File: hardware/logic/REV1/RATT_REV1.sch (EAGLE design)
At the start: 141 parts, among them IC1 MCP73832, IC10 CPC1002N, IC2 TPS2115AIPWRQ1, IC3 MAX98357, IC4 AP2112K-3.3V, IC5 PCA9539PW, IC6 TLP292-4, IC7 CPC1002N, IC8 CPC1002N, IC9 CPC1002N, J10 PHOENIX1803484, J100 RPI-ZERO, J11 PHOENIX1803484, J2 PHOENIX1803426, J3 LiPo, J4 F-1X04-SIP-100-40, J5 4P-2.0, J6 4P-2.0, J8 4P-2.0, J9 4P-2.0, Q1 DMP31D0U

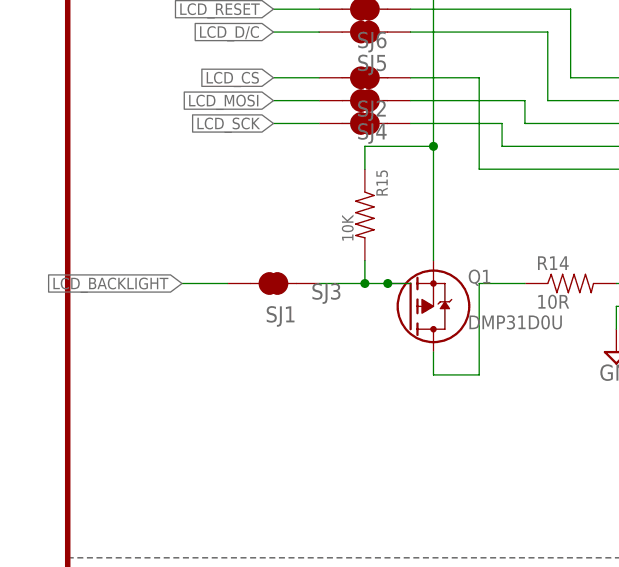
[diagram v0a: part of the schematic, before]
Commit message: REV1 as sent out to fab
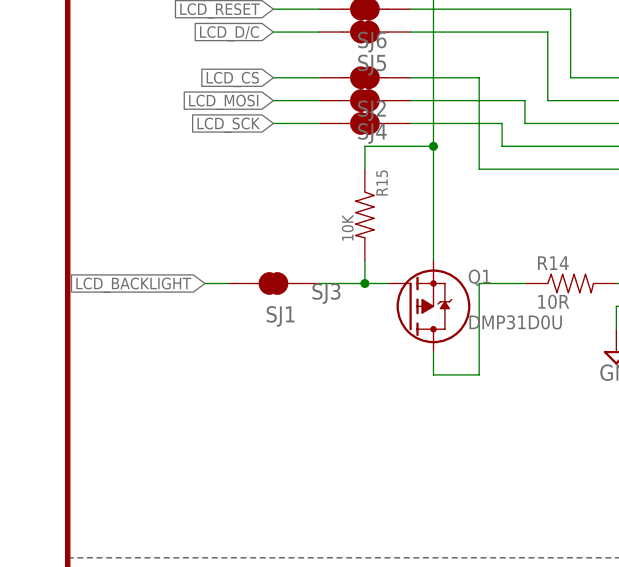
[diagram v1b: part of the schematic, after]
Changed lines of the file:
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@@
 <net name="LCD_BACKLIGHT" class="0">
 <segment>
-<wire x1="17.78" y1="99.06" x2="12.7" y2="99.06" width="0.1524" layer="91"/>
-<label x="12.7" y="99.06" size="1.27" layer="95" font="vector" rot="R180" xref="yes"/>
+<wire x1="17.78" y1="99.06" x2="15.24" y2="99.06" width="0.1524" layer="91"/>
+<label x="15.24" y="99.06" size="1.27" layer="95" font="vector" rot="R180" xref="yes"/>
 <pinref part="SJ1" gate="G$1" pin="2"/>
 </segment>
@@
 <segment>
 <pinref part="SJ1" gate="G$1" pin="1"/>
-<wire x1="38.1" y1="99.06" x2="35.56" y2="99.06" width="0.1524" layer="91"/>
 <pinref part="R15" gate="G$1" pin="2"/>
 <wire x1="35.56" y1="99.06" x2="33.02" y2="99.06" width="0.1524" layer="91"/>
@@
 <junction x="33.02" y="99.06"/>
 <pinref part="Q1" gate="G$1" pin="G"/>
-<junction x="35.56" y="99.06"/>
-</segment>
-</net>
+</segment>
+</net>
